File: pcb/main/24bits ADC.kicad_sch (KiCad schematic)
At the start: 8 parts

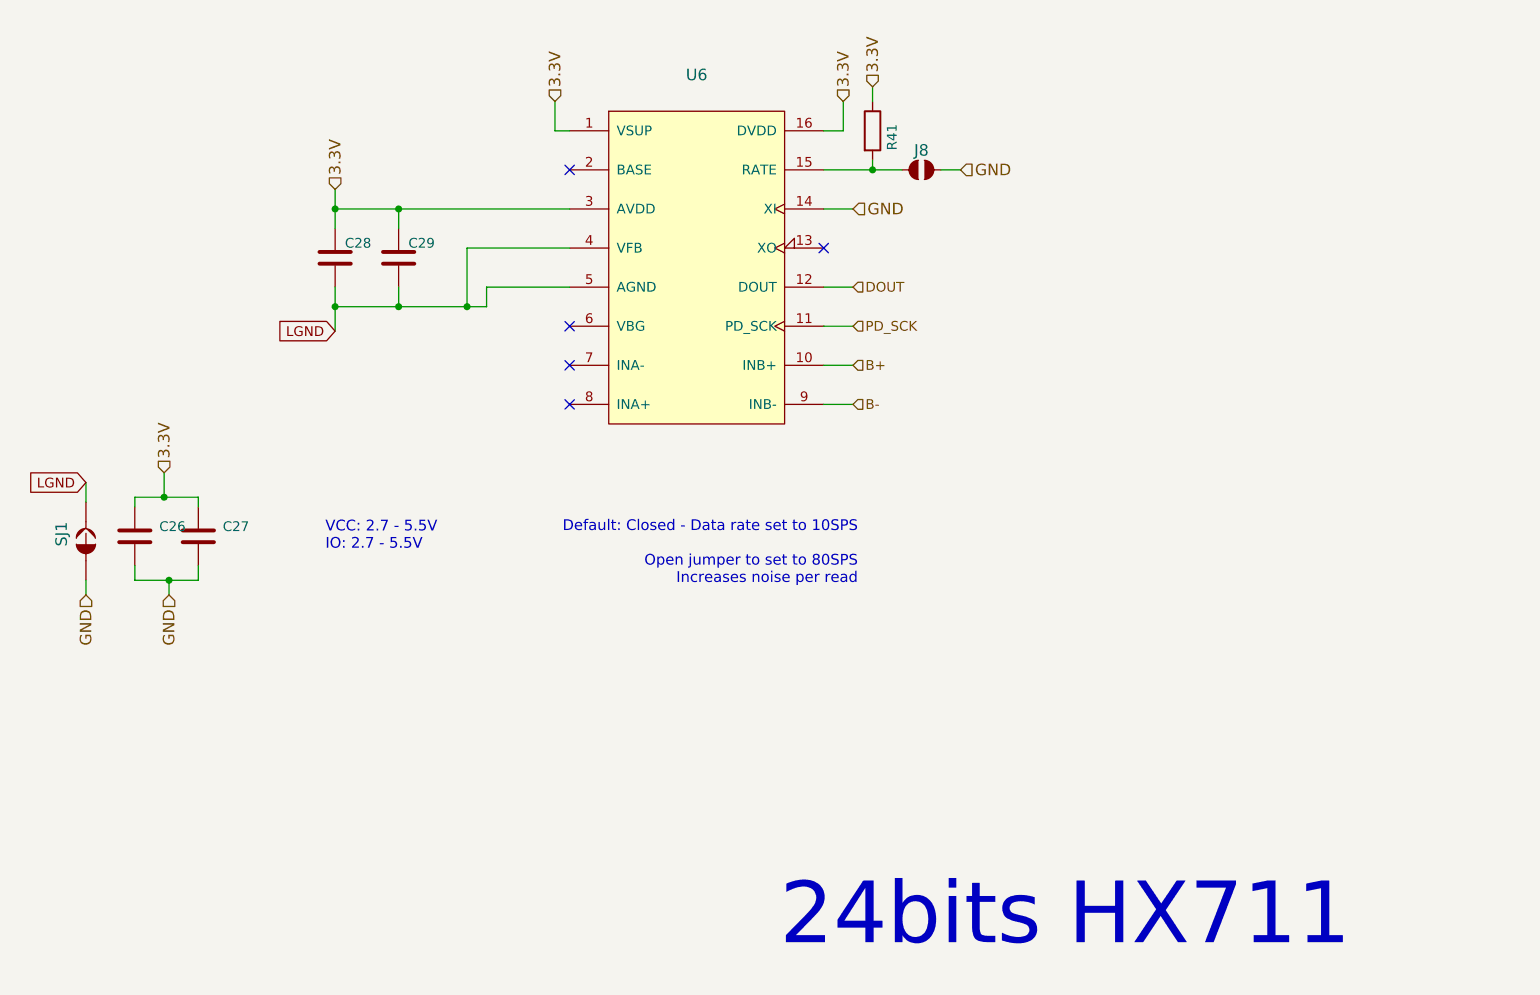
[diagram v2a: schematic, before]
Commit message: feat: updated BOM
BOM ready to order in v0.2
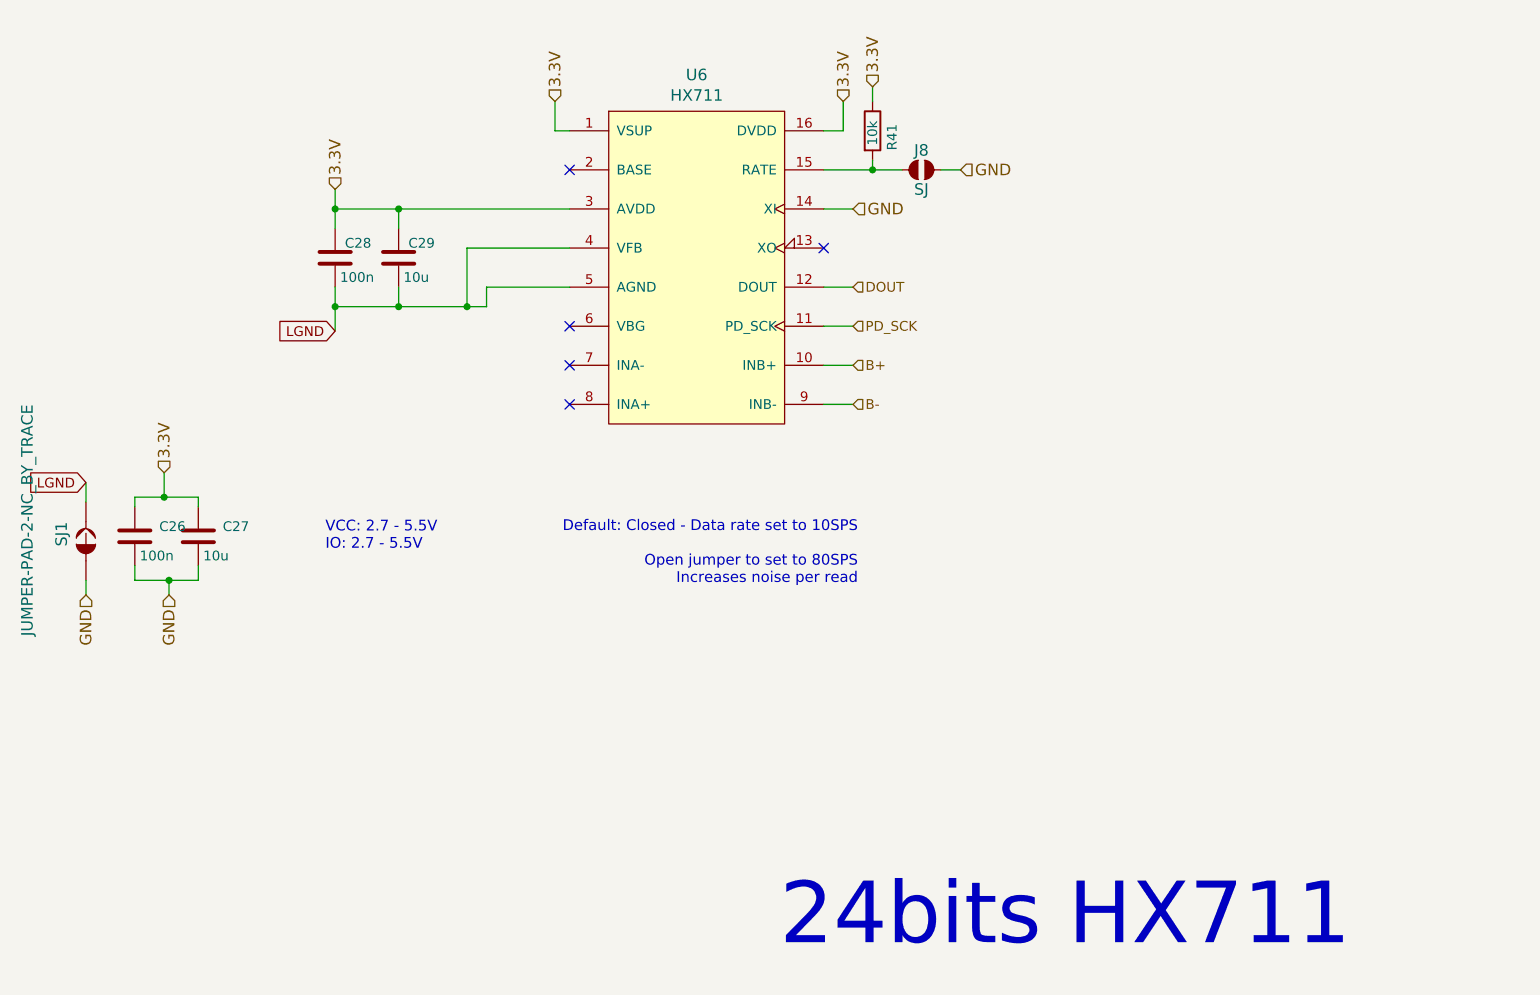
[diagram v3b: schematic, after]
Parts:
- C26, C28: value (none) -> 100n; footprint (none) -> Capacitor_SMD:C_0805_2012Metric_Pad1.18x1.45mm_HandSolder
- C27, C29: value (none) -> 10u; footprint (none) -> Capacitor_SMD:C_0805_2012Metric_Pad1.18x1.45mm_HandSolder; MFN Wurth Elektronik -> Samsung Electro-Mechanics; MFP 885012207072 -> CL21A106KOQNNNG; S1PL https://www.mouser.com/ProductDetail/Wurth-Elektronik/88501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 -> https://www.mouser.com/ProductDetail/Samsung-Electro-Mechan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; S1PN 710-885012207072 -> 187-CL21A106KOQNNNG
- J8: value (none) -> SJ; footprint (none) -> Jumper:SolderJumper-2_P1.3mm_Open_RoundedPad1.0x1.5mm
- R41: value (none) -> 10k; footprint (none) -> Resistor_SMD:R_0805_2012Metric_Pad1.20x1.40mm_HandSolder
- SJ1: value (none) -> JUMPER-PAD-2-NC_BY_TRACE; footprint (none) -> Jumper:SolderJumper-2_P1.3mm_Open_RoundedPad1.0x1.5mm
- U6: value (none) -> HX711; footprint (none) -> Package_SO:SOIC-16_3.9x9.9mm_P1.27mm
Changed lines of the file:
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@@
       (effects (font (size 1.4986 1.4986)) (justify right))
     )
-    (property "Value" "" (id 1) (at 82.55 106.68 0)
+    (property "Value" "JUMPER-PAD-2-NC_BY_TRACE" (id 1) (at 82.55 106.68 0)
       (effects (font (size 1.4986 1.4986)) (justify right))
     )
-    (property "Footprint" "" (id 2) (at 90.17 124.46 0)
+    (property "Footprint" "Jumper:SolderJumper-2_P1.3mm_Open_RoundedPad1.0x1.5mm" (id 2) (at 90.17 124.46 0)
       (effects (font (size 1.27 1.27)) hide)
     )
@@
       (effects (font (size 1.27 1.27)) (justify left))
     )
-    (property "Value" "" (id 1) (at 97.155 126.365 0)
+    (property "Value" "100n" (id 1) (at 97.155 126.365 0)
       (effects (font (size 1.27 1.27)) (justify left))
     )
-    (property "Footprint" "" (id 2) (at 97.4852 127.635 0)
+    (property "Footprint" "Capacitor_SMD:C_0805_2012Metric_Pad1.18x1.45mm_HandSolder" (id 2) (at 97.4852 127.635 0)
       (effects (font (size 1.27 1.27)) hide)
     )
@@
       (effects (font (size 1.27 1.27)) (justify left))
     )
-    (property "Value" "" (id 1) (at 105.41 126.365 0)
+    (property "Value" "10u" (id 1) (at 105.41 126.365 0)
       (effects (font (size 1.27 1.27)) (justify left))
     )
-    (property "Footprint" "" (id 2) (at 105.7402 127.635 0)
+    (property "Footprint" "Capacitor_SMD:C_0805_2012Metric_Pad1.18x1.45mm_HandSolder" (id 2) (at 105.7402 127.635 0)
       (effects (font (size 1.27 1.27)) hide)
     )
-    (property "Datasheet" "https://www.mouser.com/datasheet/2/445/885012207072-1727745.pdf" (id 3) (at 104.775 123.825 0)
+    (property "Datasheet" "https://www.mouser.com/datasheet/2/585/MLCC-1837944.pdf" (id 3) (at 104.775 123.825 0)
       (effects (font (size 1.27 1.27)) hide)
     )
-    (property "Description" "Multilayer Ceramic Capacitors MLCC - SMD/SMT WCAP-CSGP 0.1uF 0805 10% 25V MLCC " (id 4) (at 104.775 123.825 0)
+    (property "Description" "Capacitores cerámicos de capas múltiples (MLCC) - SMD/SMT 10uF+/-10% 16V X5R 2 0805 " (id 4) (at 104.775 123.825 0)
       (effects (font (size 1.27 1.27)) hide)
     )
-    (property "MFN" "Wurth Elektronik " (id 5) (at 104.775 123.825 0)
+    (property "MFN" "Samsung Electro-Mechanics " (id 5) (at 104.775 123.825 0)
       (effects (font (size 1.27 1.27)) hide)
     )
-    (property "MFP" "885012207072" (id 6) (at 104.775 123.825 0)
+    (property "MFP" "CL21A106KOQNNNG " (id 6) (at 104.775 123.825 0)
       (effects (font (size 1.27 1.27)) hide)
     )
-    (property "S1PL" "https://www.mouser.com/ProductDetail/Wurth-Elektronik/885012207072?qs=0KOYDY2FL28rQMV4504TxA%3D%3D" (id 7) (at 104.775 123.825 0)
+    (property "S1PL" "https://www.mouser.com/ProductDetail/Samsung-Electro-Mechanics/CL21A106KOQNNNG?qs=hqM3L16%252BxlcMWI7QbqH0LA%3D%3D" (id 7) (at 104.775 123.825 0)
       (effects (font (size 1.27 1.27)) hide)
     )
-    (property "S1PN" "710-885012207072 " (id 8) (at 104.775 123.825 0)
+    (property "S1PN" "187-CL21A106KOQNNNG " (id 8) (at 104.775 123.825 0)
       (effects (font (size 1.27 1.27)) hide)
     )
@@
       (effects (font (size 1.27 1.27)) (justify left))
     )
-    (property "Value" "" (id 1) (at 123.19 90.17 0)
+    (property "Value" "100n" (id 1) (at 123.19 90.17 0)
       (effects (font (size 1.27 1.27)) (justify left))
     )
-    (property "Footprint" "" (id 2) (at 123.5202 91.44 0)
+    (property "Footprint" "Capacitor_SMD:C_0805_2012Metric_Pad1.18x1.45mm_HandSolder" (id 2) (at 123.5202 91.44 0)
       (effects (font (size 1.27 1.27)) hide)
     )
@@
       (effects (font (size 1.27 1.27)) (justify left))
     )
-    (property "Value" "" (id 1) (at 131.445 90.17 0)
+    (property "Value" "10u" (id 1) (at 131.445 90.17 0)
       (effects (font (size 1.27 1.27)) (justify left))
     )
-    (property "Footprint" "" (id 2) (at 131.7752 91.44 0)
+    (property "Footprint" "Capacitor_SMD:C_0805_2012Metric_Pad1.18x1.45mm_HandSolder" (id 2) (at 131.7752 91.44 0)
       (effects (font (size 1.27 1.27)) hide)
     )
-    (property "Datasheet" "https://www.mouser.com/datasheet/2/445/885012207072-1727745.pdf" (id 3) (at 130.81 87.63 0)
+    (property "Datasheet" "https://www.mouser.com/datasheet/2/585/MLCC-1837944.pdf" (id 3) (at 130.81 87.63 0)
       (effects (font (size 1.27 1.27)) hide)
     )
-    (property "Description" "Multilayer Ceramic Capacitors MLCC - SMD/SMT WCAP-CSGP 0.1uF 0805 10% 25V MLCC " (id 4) (at 130.81 87.63 0)
+    (property "Description" "Capacitores cerámicos de capas múltiples (MLCC) - SMD/SMT 10uF+/-10% 16V X5R 2 0805 " (id 4) (at 130.81 87.63 0)
       (effects (font (size 1.27 1.27)) hide)
     )
-    (property "MFN" "Wurth Elektronik " (id 5) (at 130.81 87.63 0)
+    (property "MFN" "Samsung Electro-Mechanics " (id 5) (at 130.81 87.63 0)
       (effects (font (size 1.27 1.27)) hide)
     )
-    (property "MFP" "885012207072" (id 6) (at 130.81 87.63 0)
+    (property "MFP" "CL21A106KOQNNNG " (id 6) (at 130.81 87.63 0)
       (effects (font (size 1.27 1.27)) hide)
     )
-    (property "S1PL" "https://www.mouser.com/ProductDetail/Wurth-Elektronik/885012207072?qs=0KOYDY2FL28rQMV4504TxA%3D%3D" (id 7) (at 130.81 87.63 0)
+    (property "S1PL" "https://www.mouser.com/ProductDetail/Samsung-Electro-Mechanics/CL21A106KOQNNNG?qs=hqM3L16%252BxlcMWI7QbqH0LA%3D%3D" (id 7) (at 130.81 87.63 0)
       (effects (font (size 1.27 1.27)) hide)
     )
-    (property "S1PN" "710-885012207072 " (id 8) (at 130.81 87.63 0)
+    (property "S1PN" "187-CL21A106KOQNNNG " (id 8) (at 130.81 87.63 0)
       (effects (font (size 1.27 1.27)) hide)
     )
@@
       (effects (font (size 1.4986 1.4986)))
     )
-    (property "Value" "" (id 1) (at 198.755 78.74 0)
+    (property "Value" "SJ" (id 1) (at 198.755 78.74 0)
       (effects (font (size 1.4986 1.4986)))
     )
-    (property "Footprint" "" (id 2) (at 198.755 76.2 0)
+    (property "Footprint" "Jumper:SolderJumper-2_P1.3mm_Open_RoundedPad1.0x1.5mm" (id 2) (at 198.755 76.2 0)
       (effects (font (size 1.27 1.27)) hide)
     )
@@
       (effects (font (size 1.27 1.27)) (justify left))
     )
-    (property "Value" "" (id 1) (at 192.405 73.025 90)
+    (property "Value" "10k" (id 1) (at 192.405 73.025 90)
       (effects (font (size 1.27 1.27)) (justify left))
     )
-    (property "Footprint" "" (id 2) (at 190.627 71.12 90)
+    (property "Footprint" "Resistor_SMD:R_0805_2012Metric_Pad1.20x1.40mm_HandSolder" (id 2) (at 190.627 71.12 90)
       (effects (font (size 1.27 1.27)) hide)
     )
@@
       (effects (font (size 1.4986 1.4986)))
     )
-    (property "Value" "" (id 1) (at 169.545 66.5226 0)
+    (property "Value" "HX711" (id 1) (at 169.545 66.5226 0)
       (effects (font (size 1.4986 1.4986)))
     )
-    (property "Footprint" "" (id 2) (at 170.815 115.57 0)
+    (property "Footprint" "Package_SO:SOIC-16_3.9x9.9mm_P1.27mm" (id 2) (at 170.815 115.57 0)
       (effects (font (size 1.27 1.27)) hide)
     )
